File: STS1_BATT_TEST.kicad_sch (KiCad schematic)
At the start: 6 parts, among them J1 TE 282834-6, J2 Conn_01x15

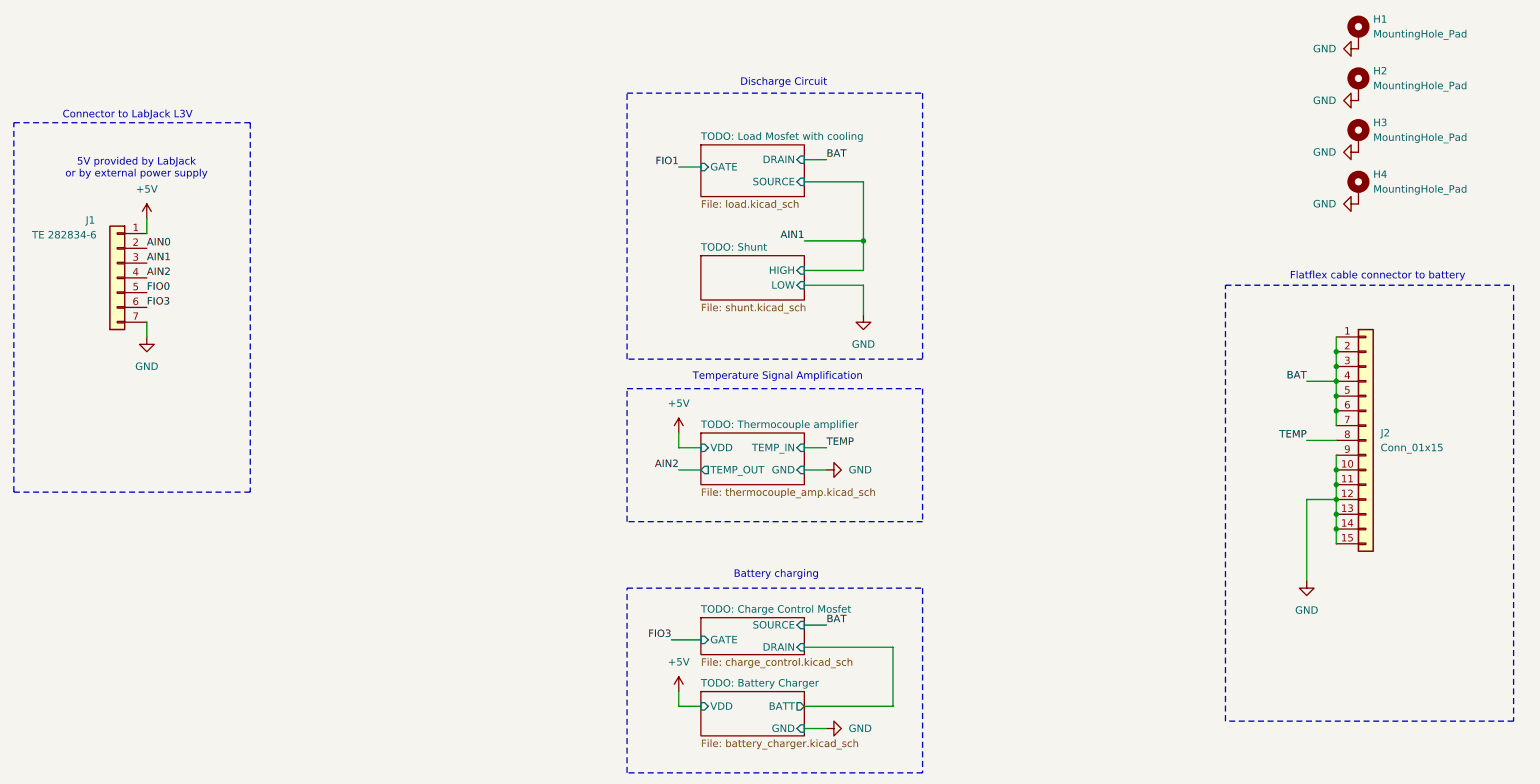
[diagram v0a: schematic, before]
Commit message: Prepared STS1_BATT_TEST.
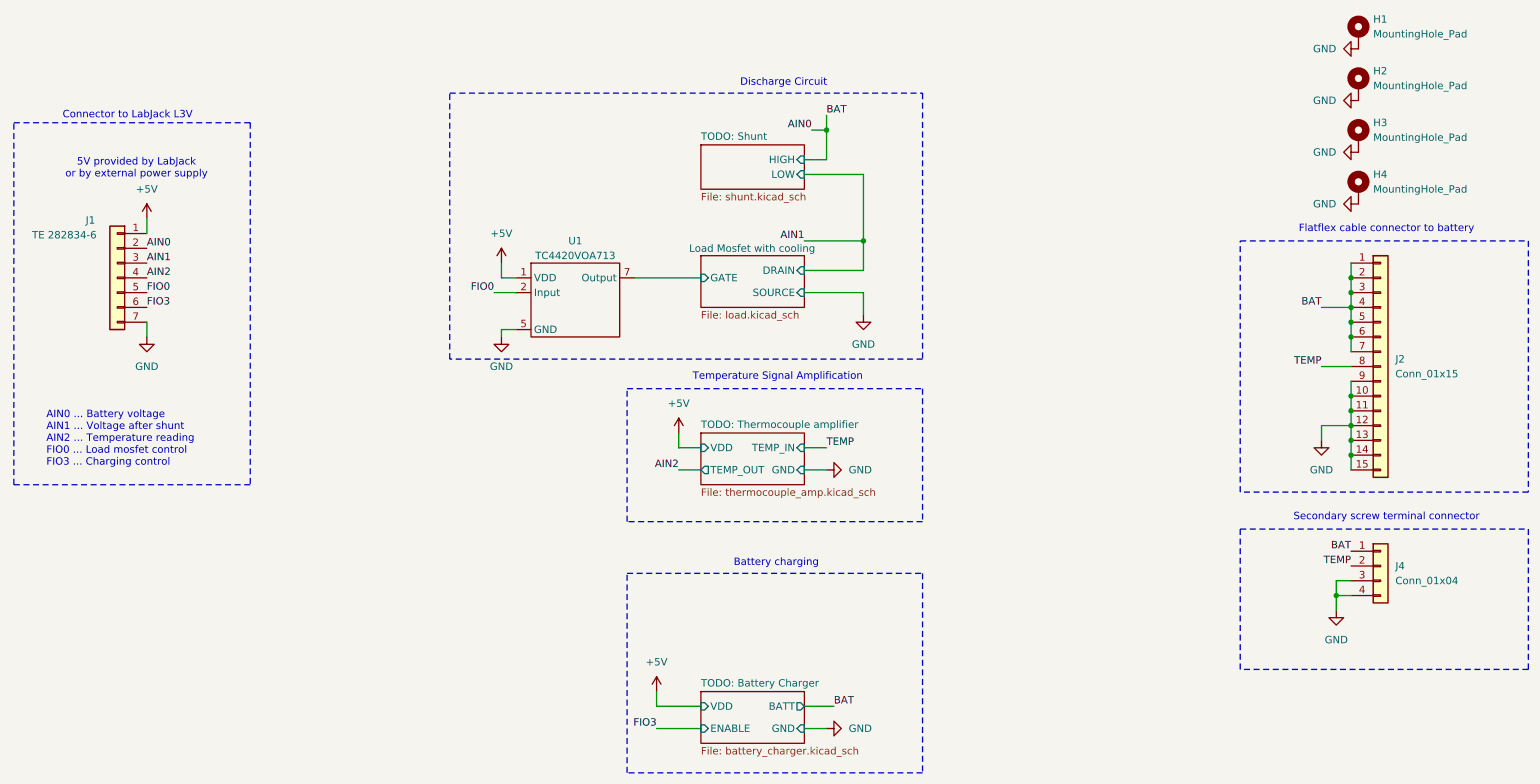
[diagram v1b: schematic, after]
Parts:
- added J4: Conn_01x04, STS1_Connectors:TE_282834-4, symbol Connector_Generic:Conn_01x04
- added U1: TC4420VOA713, Package_SO:SOIC-8_5.275x5.275mm_P1.27mm, symbol STS_Transistor_FET:TC4420
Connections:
- net BAT is gone; now on net AIN0: J2.1 (Pin_1), J2.2 (Pin_2), J2.3 (Pin_3), J2.4 (Pin_4), J2.5 (Pin_5), J2.6 (Pin_6), J2.7 (Pin_7)
- net +5V: now also U1.1 (VDD), U1.8 (VDD)
- net AIN0: now also J4.1 (Pin_1)
- net FIO0: now also U1.2 (Input)
- net GND: now also J4.3 (Pin_3), J4.4 (Pin_4), U1.4 (GND), U1.5 (GND)
- net TEMP: now also J4.2 (Pin_2)
- new net Load Mosfet with cooling/GATE: U1.6 (Output), U1.7 (Output)
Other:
- sheet TODO: Load Mosfet with cooling renamed Load Mosfet with cooling
- removed sheet TODO: Charge Control Mosfet
- sheet TODO: Battery Charger ports: added ENABLE; removed none
- note added: "AIN0 ... Battery voltage AIN1 ... Voltage after shunt AIN2 ... Temperature reading FIO0 ... Load mosfet control FIO3 ... Charging control"
- note added: "Secondary screw terminal connector"
- moved on the sheet: J2
